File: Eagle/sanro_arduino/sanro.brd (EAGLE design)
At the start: 50.8 x 37.8 mm, 5 parts

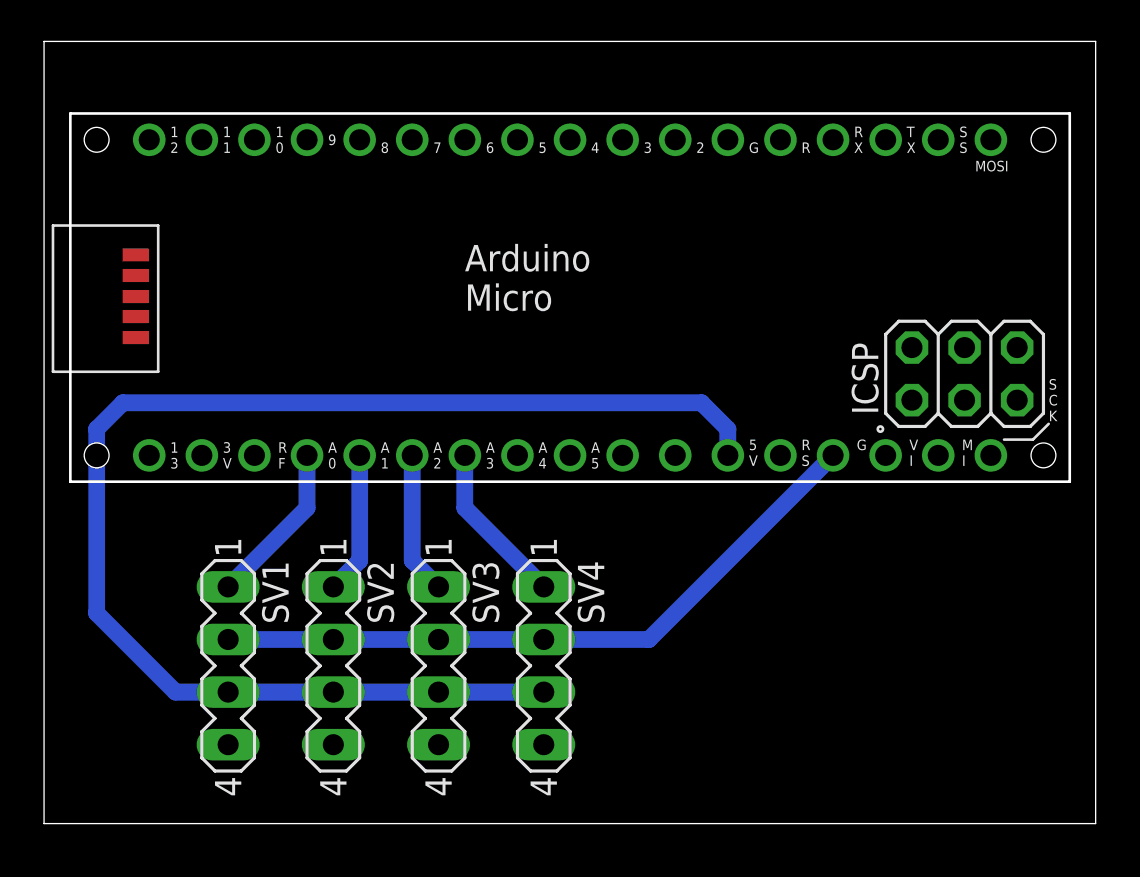
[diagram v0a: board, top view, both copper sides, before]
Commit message: Upload EPS file for the PCB
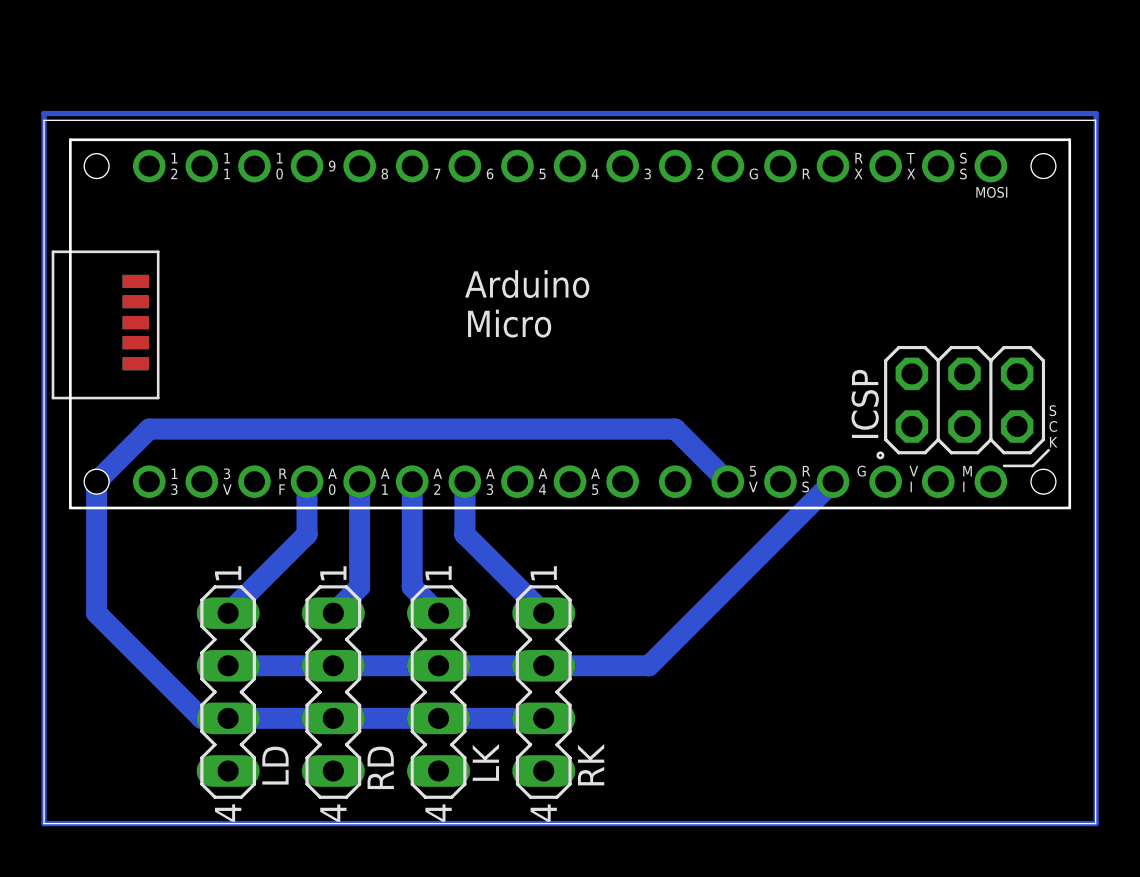
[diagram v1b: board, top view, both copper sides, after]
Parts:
- removed SV1, SV2, SV3, SV4: (no value), con-lstb:MA04-1
- added LD, LK, RD, RK: (no value), con-lstb:MA04-1
- moved PCB1 1.27 mm to (1.27, 15.2)
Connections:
- net N$1: now also LD.1; no longer SV1.1
- net N$2: now also RD.1; no longer SV2.1
- net N$3: now also LK.1; no longer SV3.1
- net N$4: now also RK.1; no longer SV4.1
- net N$5: now also LD.2, LK.2, RD.2, RK.2; no longer SV1.2, SV2.2, SV3.2, SV4.2
- net N$6: now also LD.3, LK.3, RD.3, RK.3; no longer SV1.3, SV2.3, SV3.3, SV4.3
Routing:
- net N$7: track 0.00 -> 170.2 mm
- net N$6: track 64.9 -> 62.6 mm
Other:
- board size 50.8 x 37.8 mm -> 50.8 x 34 mm
